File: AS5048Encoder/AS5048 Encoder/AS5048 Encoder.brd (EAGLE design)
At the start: 43.1 x 39.9 mm, 6 parts

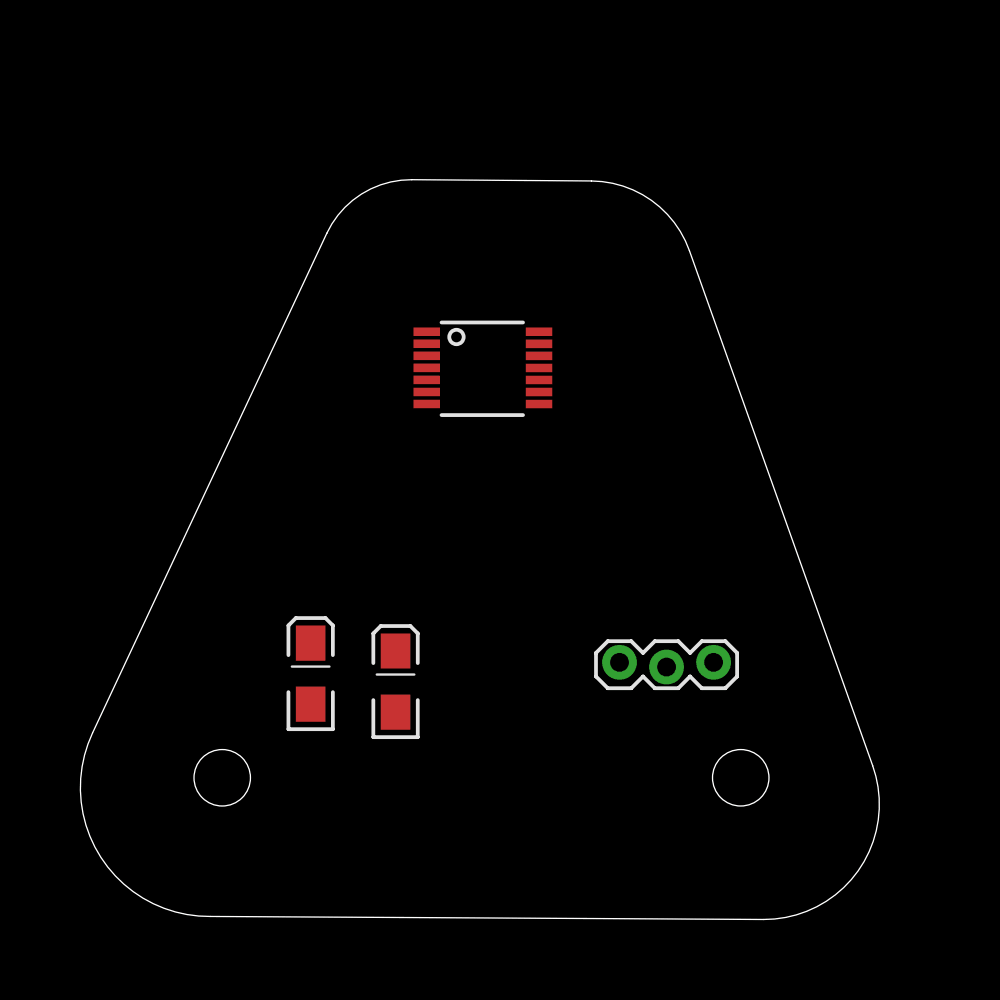
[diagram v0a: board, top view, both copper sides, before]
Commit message: pre route
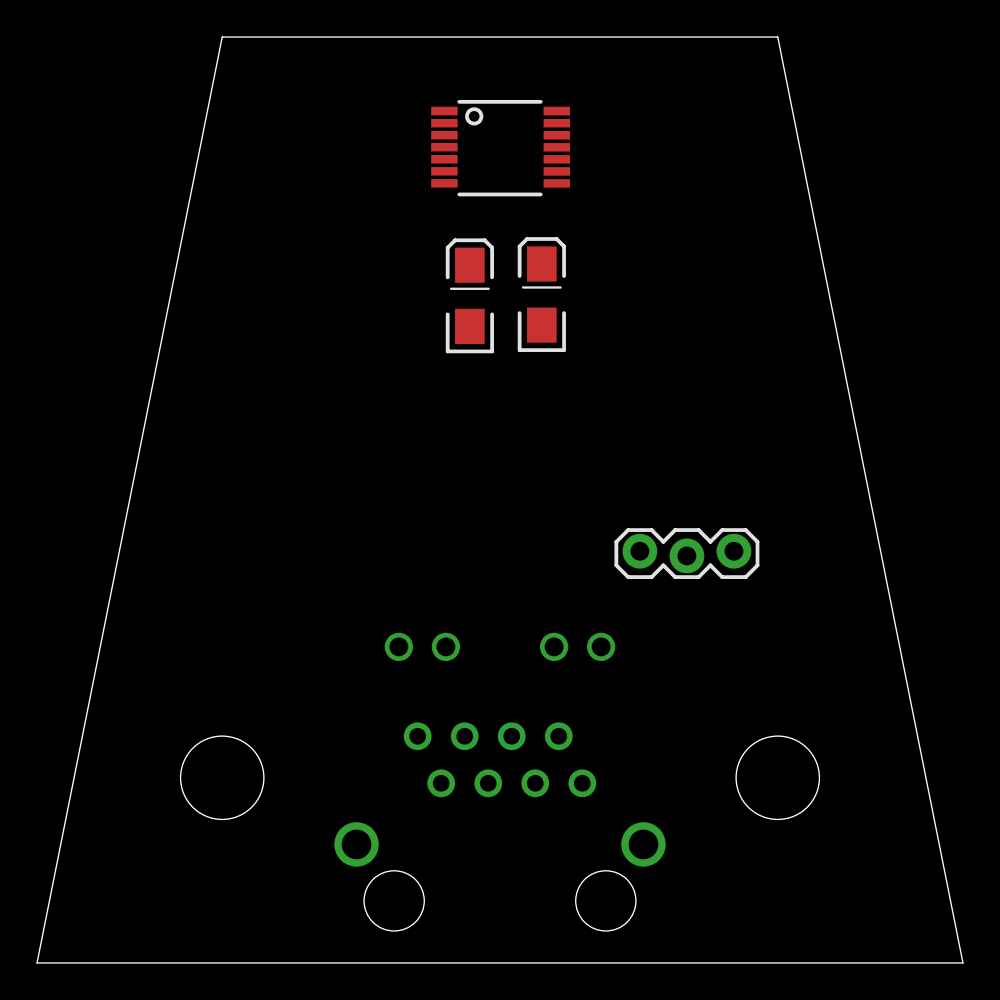
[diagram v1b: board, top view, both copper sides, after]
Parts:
- removed U$2, U$3: (no value), SparkFun-Electromechanical:STAND-OFF-TIGHT
- added X1: SI-50170, con-stewart:SI-50170
- moved C3 22.3 mm to (27.3, 36.1)
- moved C4 22.1 mm to (23.4, 36.0)
- moved U$1 12.0 mm to (25.0, 44.0)
- moved JP1 6.10 mm to (32.6, 22.1)
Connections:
- net GND: now also X1.3
- net PWM: now also X1.2
- net VCC: now also X1.1
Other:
- board size 43.1 x 39.9 mm -> 50 x 50 mm
